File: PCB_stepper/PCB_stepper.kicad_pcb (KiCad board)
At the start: 2 copper layers, 70 x 48.2 mm, 47 parts, among them J1 USB_C_Receptacle_USB2.0, J2 CON_CAN, J3 CON_CAN, J4 12V, J5 Conn_01x04_Male, SW1 RST, SW2 BOOT, U1 STM32F302C6Tx, U2 SN65HVD232, U3 NCP1117-3.3_SOT223, Y1 8MHz

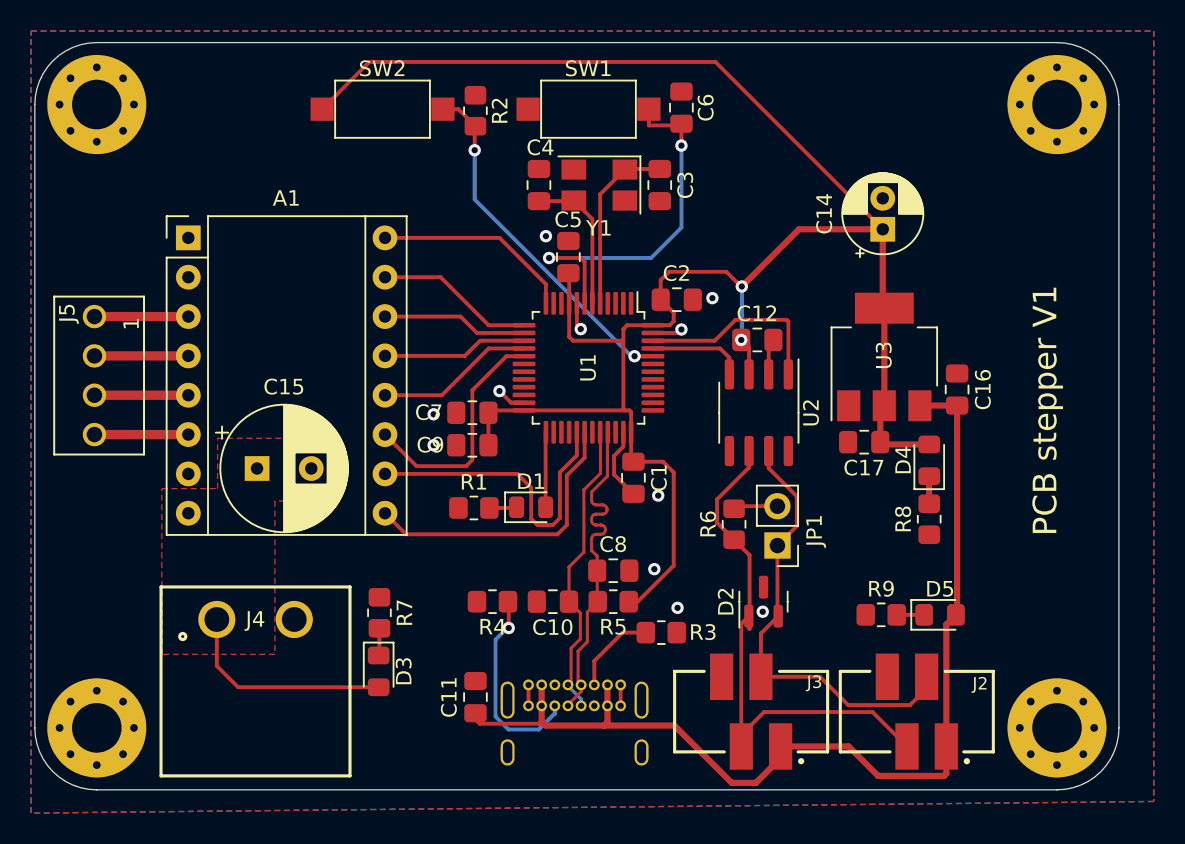
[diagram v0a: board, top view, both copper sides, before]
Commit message: MAJ principal + stepper
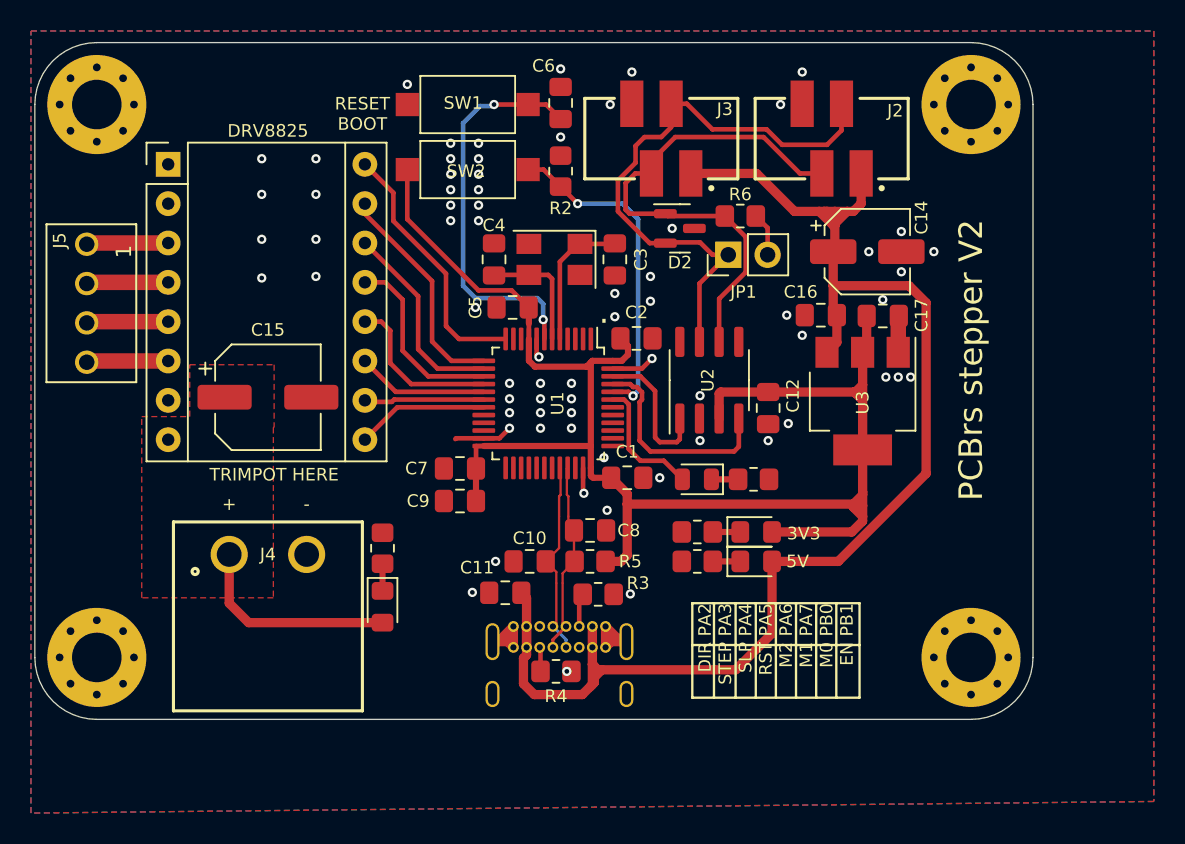
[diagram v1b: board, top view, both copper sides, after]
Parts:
- C14: footprint Capacitor_THT:CP_Radial_D5.0mm_P2.00mm -> Capacitor_SMD:CP_Elec_5x5.4
- C15: value 100u -> 47u; footprint Capacitor_THT:CP_Radial_D8.0mm_P3.50mm -> Capacitor_SMD:CP_Elec_6.3x5.4
- C6: value 0.1u -> 100n
- moved J3 37.5 mm to (148.7, 62.2)
- moved J2 37.4 mm to (159.7, 62.2)
- moved D2 24.7 mm to (149.9, 68.0), turned to 0 degrees
- moved R6 19.9 mm to (153.8, 67.2), turned to 0 degrees
- moved JP1 19.0 mm to (153.0, 69.7), turned to 90 degrees
- moved R1 18.2 mm to (154.7, 84.2), turned to 180 degrees
- moved R8 15.0 mm to (151.0, 87.6), turned to 0 degrees
- moved D5 12.4 mm to (154.8, 89.5)
- moved R9 12.4 mm to (151.0, 89.5)
- moved D4 12.1 mm to (154.8, 87.6), turned to 0 degrees
- moved D1 10.9 mm to (151.0, 84.2), turned to 180 degrees
- moved C16 10.0 mm to (159.0, 73.6), turned to 180 degrees
- moved C17 8.24 mm to (163.0, 73.7), turned to 0 degrees
- moved C6 7.81 mm to (142.2, 59.9)
- moved SW1 7.81 mm to (136.2, 60.0)
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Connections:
- C14 pad 1: +3V3 -> +5V
- D1 pad 2: Net-(D1-Pad2) -> /USR_LED
- U1 pad 18: unconnected-(U1-Pad18) -> /M0
- U1 pad 19: unconnected-(U1-Pad19) -> /EN
- U1 pad 21: /USART3_TX -> unconnected-(U1-Pad21)
- U1 pad 22: /USART3_RX -> unconnected-(U1-Pad22)
- U1 pad 25: Net-(D1-Pad2) -> unconnected-(U1-Pad25)
- U1 pad 29: /M0 -> unconnected-(U1-Pad29)
- U1 pad 30: /EN -> unconnected-(U1-Pad30)
- U1 pad 43: unconnected-(U1-Pad43) -> /USR_LED
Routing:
- net +3V3: track 128.7 -> 101.6 mm, vias 2 -> 0
- net +5V: track 66.4 -> 93.1 mm
- net /M0: track 20.0 -> 7.78 mm
- net Net-(J1-PadB5): track 12.9 -> 1.57 mm, vias 1 -> 0
- net /EN: track 19.0 -> 8.54 mm
- net /USB+: track 21.9 -> 12.6 mm
- net /CANH: track 29.0 -> 37.9 mm
- net /USR_LED: track 0.00 -> 8.33 mm
- net /CANRX: track 6.26 -> 13.9 mm
- net /M1: track 15.4 -> 8.50 mm
- net /USB-: track 19.5 -> 12.7 mm
- net GND: track 15.4 -> 21.1 mm, vias 11 -> 69
- net Net-(D1-Pad2): track 4.85 -> 0.00 mm
- net /STEP: track 10.3 -> 14.6 mm
- net /DIR: track 12.9 -> 16.8 mm
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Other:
- board size 70 x 48.2 mm -> 64.4 x 43.7 mm
- board text added: "+"
- board text added: "-"
- board text added: "."
- board text added: "3V3"
- board text added: "5V"
- board text added: "DIR PA2 STEP PA3 SLP PA4 RST PA5 M2 PA6 M1 PA7 M0 PB0 EN PB1"
- board text added: "DRV8825"
- board text added: "PCBrs stepper V2"
- board text added: "RESET BOOT"
- board text added: "TRIMPOT HERE"
- board text removed: "PCB stepper V1"
